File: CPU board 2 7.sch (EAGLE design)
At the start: 59 parts, among them U1 74HC245, U10 74HC08, U11 74HC32, U12 SST39SF010, U13 AS6C62256, U14 SST39SF010, U15 SST39SF010, U2 74HC245, U3 74HC245, U4 TL7705, U6 74HC138, U7 74HC74, U8 74HC11, U9 74HC02

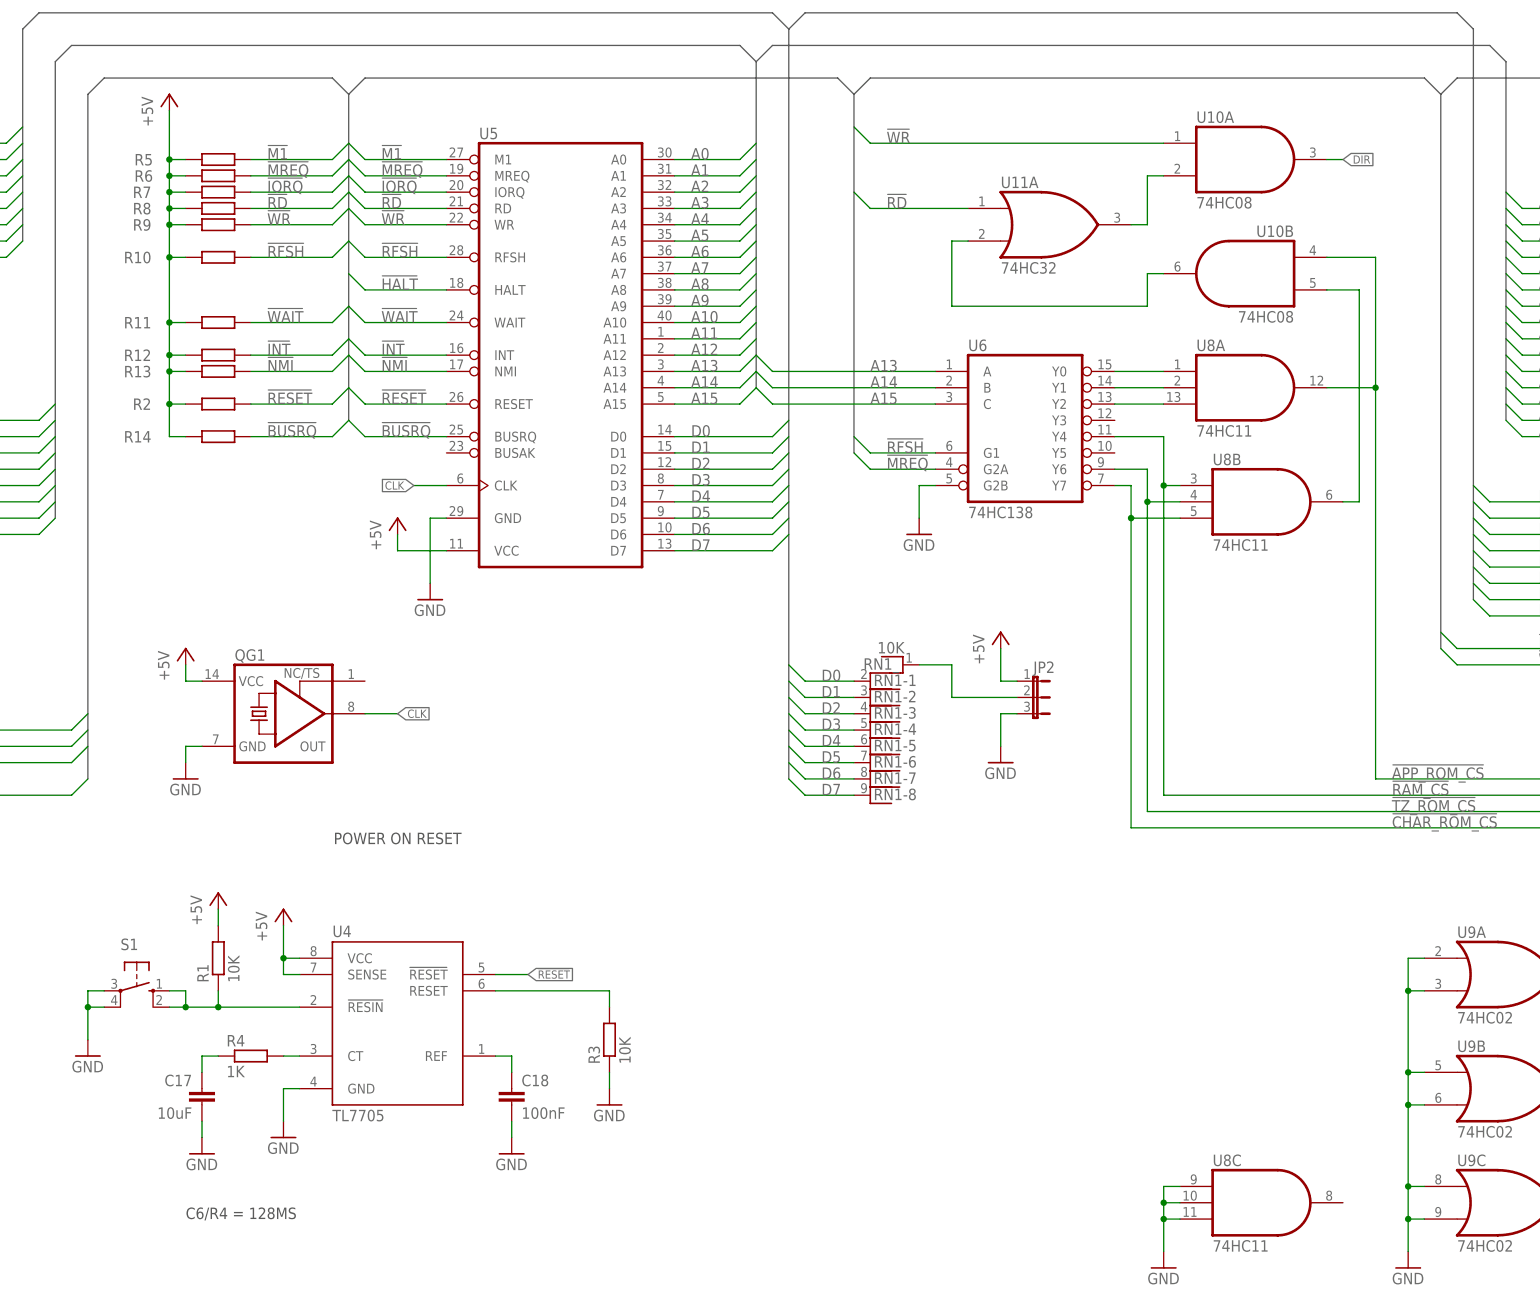
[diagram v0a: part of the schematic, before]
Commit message: Slight re-arrangement
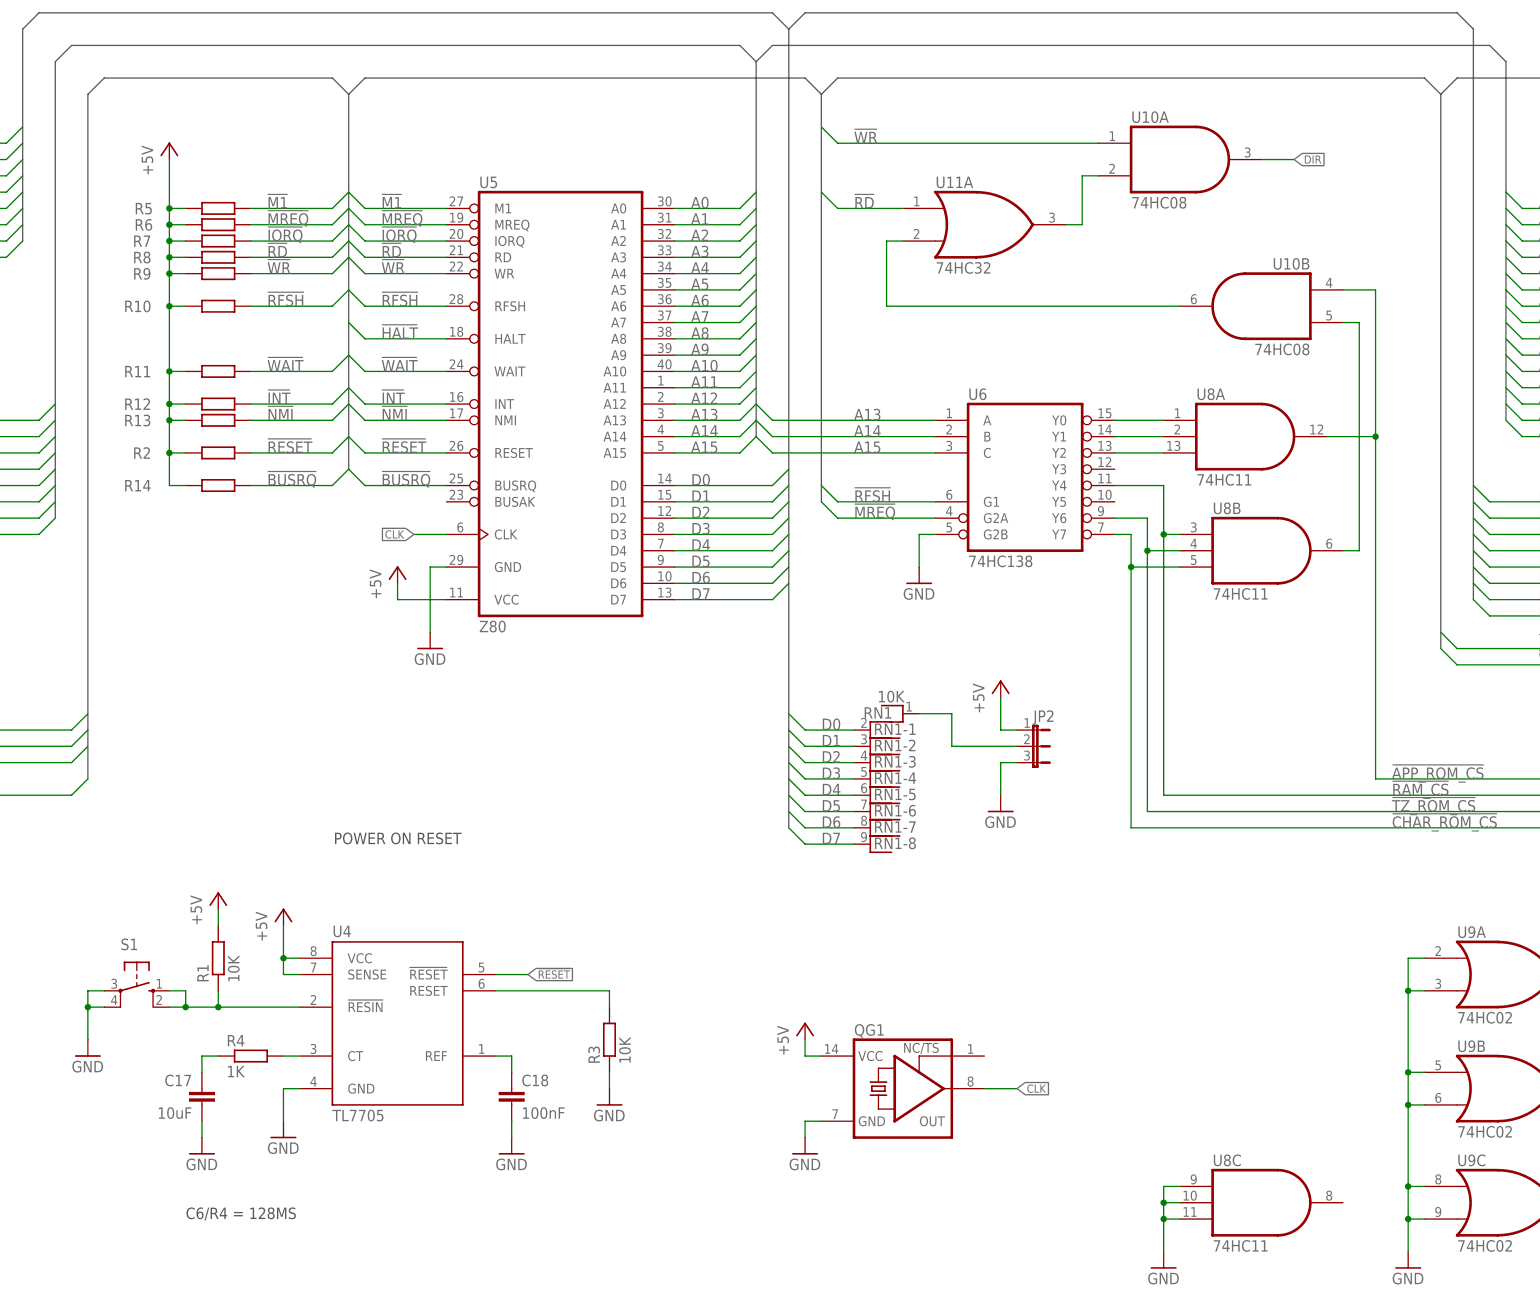
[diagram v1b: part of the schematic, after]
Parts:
- U5: value (none) -> Z80
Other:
- moved on the sheet: JP2, QG1, R10, R11, R12, R13, R14, R2, R5, R6, R7, R8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
